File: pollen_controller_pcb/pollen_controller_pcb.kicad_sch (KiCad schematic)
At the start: 15 parts, among them J1 Conn_02x20_Odd_Even, J2 Motor focus, J3 Motor tape, J4 Focus sensor, J5 Lights, J6 Power in, J7 GPS, U1 ULN2003, U2 ULN2003, U3 NB-IOT-BC660, U4 AM2302

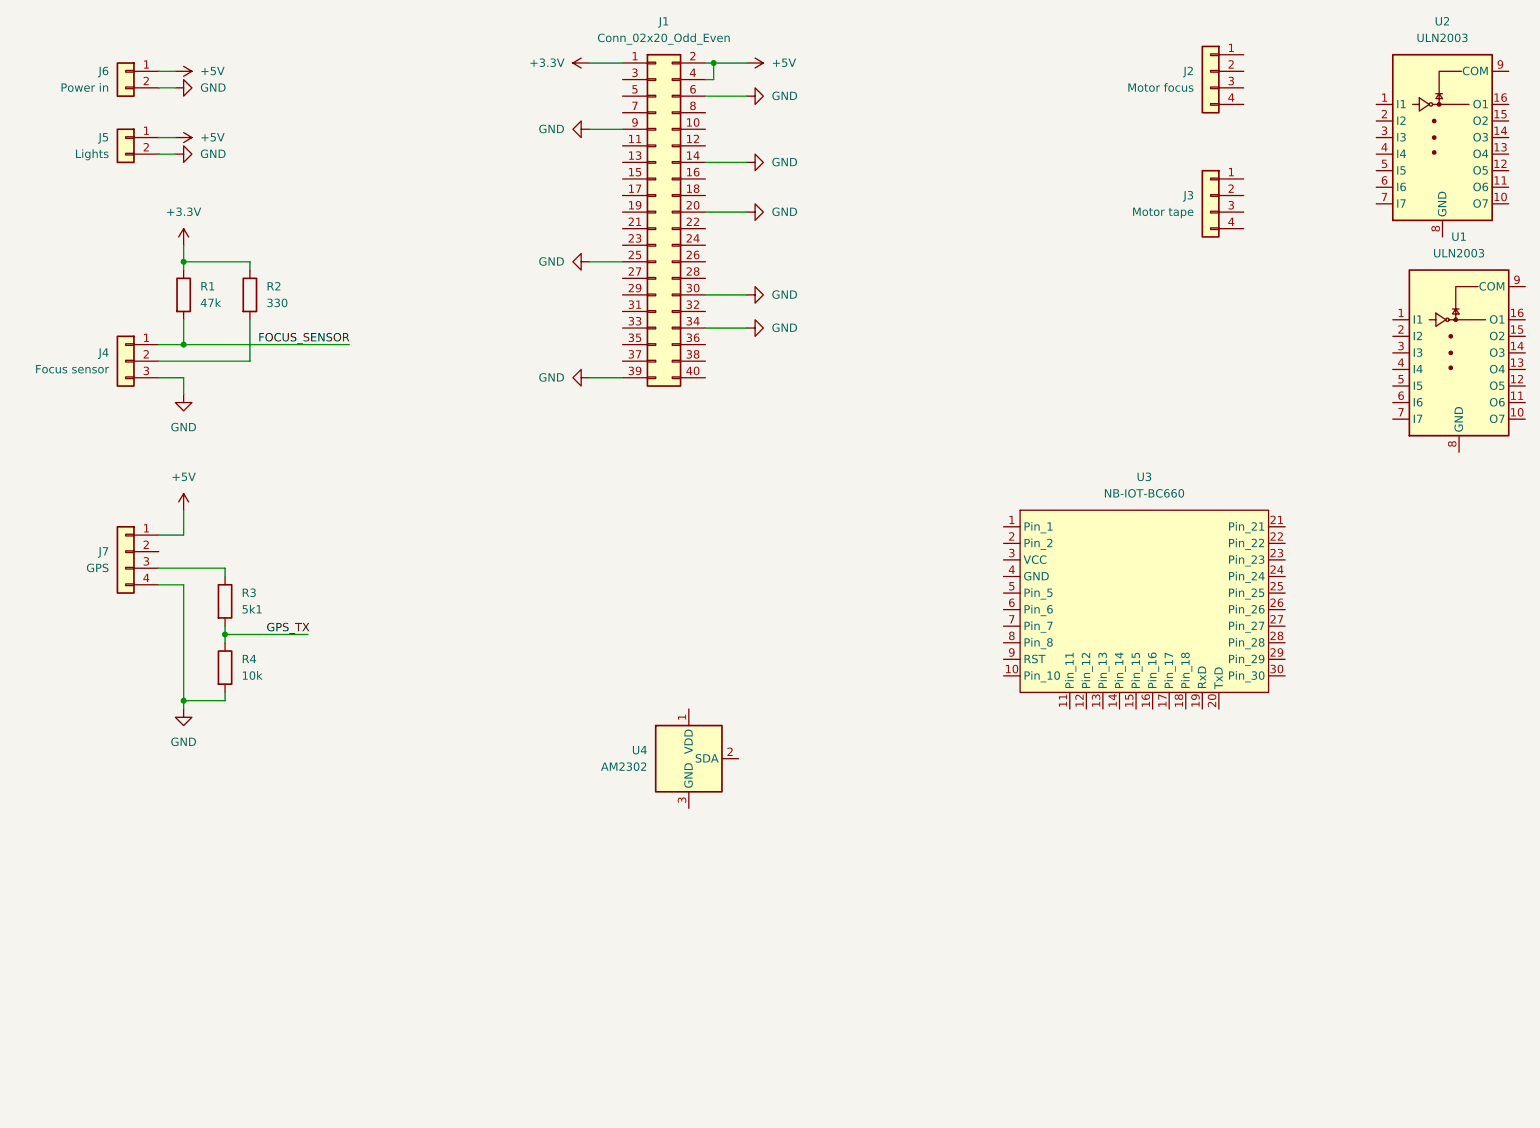
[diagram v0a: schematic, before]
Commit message: PCB changes
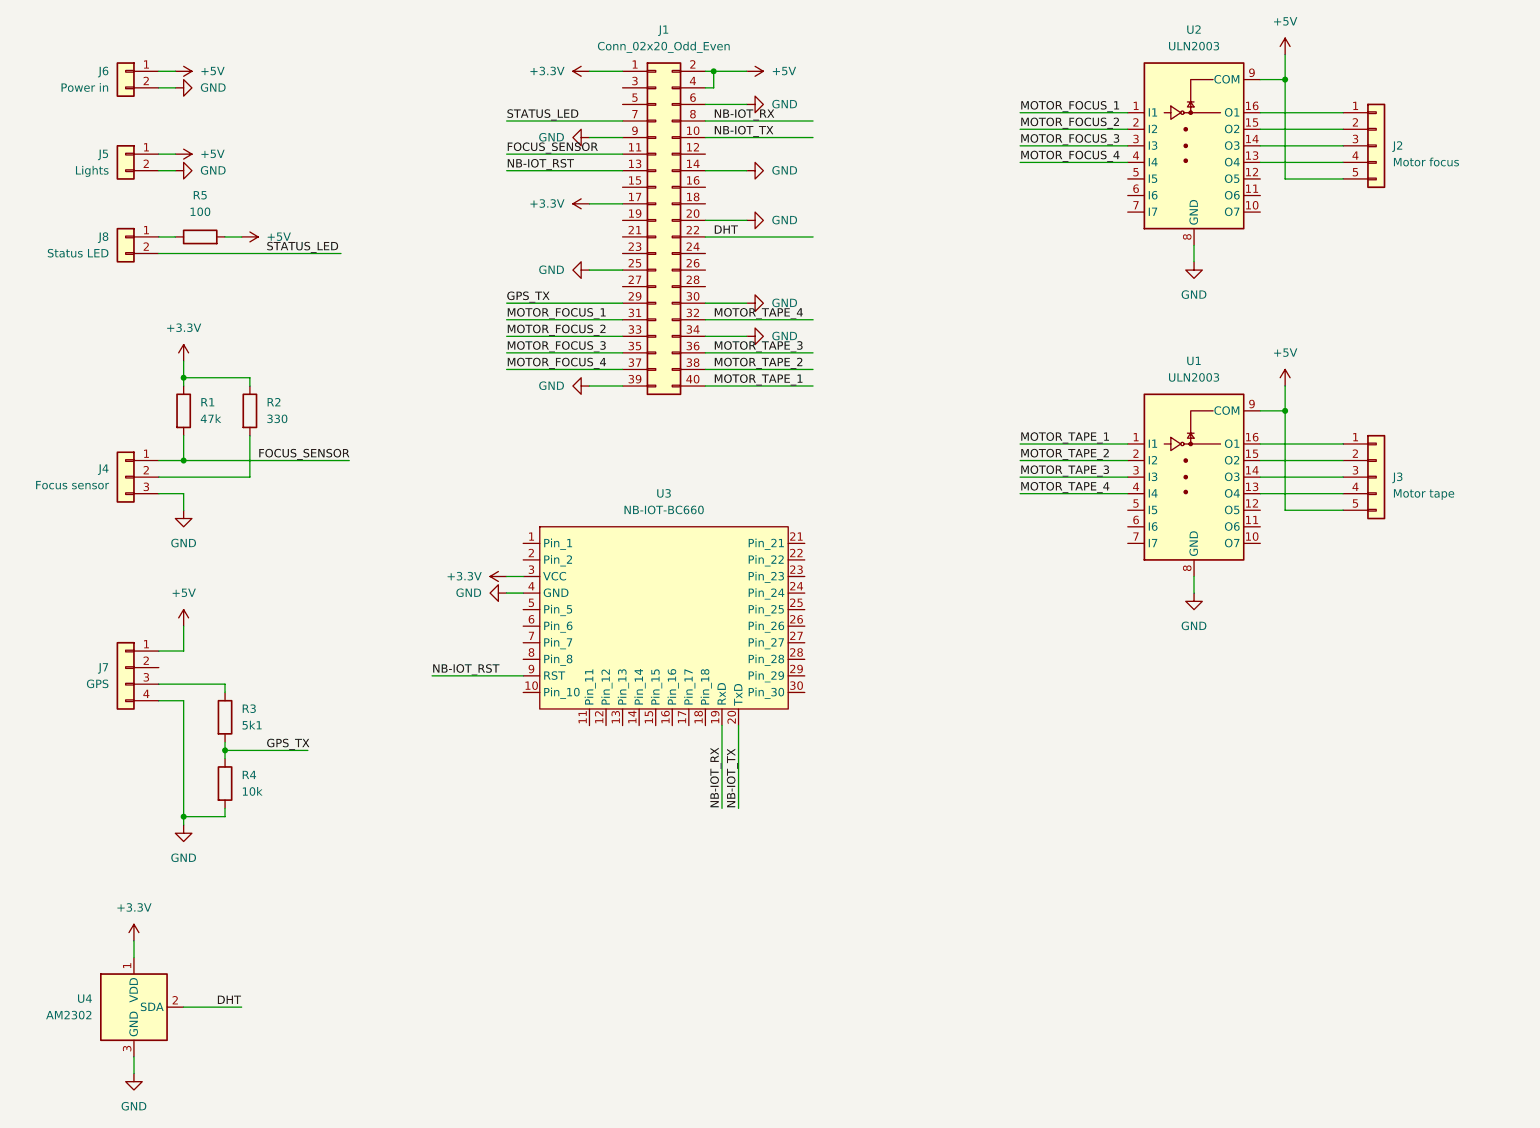
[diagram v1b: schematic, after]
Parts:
- added J8: Status LED, Connector_PinSocket_2.54mm:PinSocket_1x02_P2.54mm_Vertical, symbol Connector_Generic:Conn_01x02
- added R5: 100, Resistor_THT:R_Axial_DIN0207_L6.3mm_D2.5mm_P10.16mm_Horizontal, symbol Device:R
- J2, J3: footprint Connector_PinHeader_2.54mm:PinHeader_1x04_P2.54mm_Vertical -> Connector_PinHeader_2.54mm:PinHeader_1x05_P2.54mm_Vertical; symbol Connector_Generic:Conn_01x04 -> Connector_Generic:Conn_01x05
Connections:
- net +3.3V: now also J1.17 (Pin_17), U3.3 (VCC), U4.1 (VDD)
- net +5V: now also J2.5 (Pin_5), J3.5 (Pin_5), U1.9 (COM), U2.9 (COM), R5.2
- net FOCUS_SENSOR: now also J1.11 (Pin_11)
- net GND: now also U1.8 (GND), U2.8 (GND), U3.4 (GND), U4.3 (GND), U4.4 (GND)
- net GPS_TX: now also J1.29 (Pin_29)
- net DHT: now reaches U4.2 (SDA)
- net DHT: now also J1.22 (Pin_22)
- net MOTOR_FOCUS_1: now reaches U2.1 (I1)
- net MOTOR_FOCUS_1: now also J1.31 (Pin_31)
- net at U2.13 (O4): now also J2.4 (Pin_4)
- net at U2.14 (O3): now also J2.3 (Pin_3)
- net at U2.15 (O2): now also J2.2 (Pin_2)
- net at U2.16 (O1): now also J2.1 (Pin_1)
- net MOTOR_FOCUS_2: now reaches U2.2 (I2)
- net MOTOR_FOCUS_2: now also J1.33 (Pin_33)
- net MOTOR_FOCUS_3: now reaches U2.3 (I3)
- net MOTOR_FOCUS_3: now also J1.35 (Pin_35)
- net MOTOR_FOCUS_4: now reaches U2.4 (I4)
- net MOTOR_FOCUS_4: now also J1.37 (Pin_37)
- net MOTOR_TAPE_1: now reaches U1.1 (I1)
- net MOTOR_TAPE_1: now also J1.40 (Pin_40)
- net at U1.13 (O4): now also J3.4 (Pin_4)
- net at U1.14 (O3): now also J3.3 (Pin_3)
- net at U1.15 (O2): now also J3.2 (Pin_2)
- net at U1.16 (O1): now also J3.1 (Pin_1)
- net MOTOR_TAPE_2: now reaches U1.2 (I2)
- net MOTOR_TAPE_2: now also J1.38 (Pin_38)
- net MOTOR_TAPE_3: now reaches U1.3 (I3)
- net MOTOR_TAPE_3: now also J1.36 (Pin_36)
- net MOTOR_TAPE_4: now reaches U1.4 (I4)
- net MOTOR_TAPE_4: now also J1.32 (Pin_32)
- net NB-IOT_TX: now reaches J1.10 (Pin_10)
- net NB-IOT_TX: now also U3.20 (TxD)
- net NB-IOT_RST: now reaches J1.13 (Pin_13)
- net NB-IOT_RST: now also U3.9 (RST)
- net STATUS_LED: now reaches J1.7 (Pin_7)
- net STATUS_LED: now also J8.2 (Pin_2)
- net NB-IOT_RX: now reaches J1.8 (Pin_8)
- net NB-IOT_RX: now also U3.19 (RxD)
- new net: J8.1 (Pin_1), R5.1
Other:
- moved on the sheet: J1, J4, J5, J7, R1, R2, R3, R4, U1, U2, U3, U4
